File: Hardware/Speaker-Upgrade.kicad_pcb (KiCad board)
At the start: 2 copper layers, 130.2 x 56.5 mm, 33 parts, among them J1 POWER, J2 CONN_PCB1, J3 CONN_PCB2, J4 AUDIO_JACK, U1 LM7805, U2 WIN-668, U3 AN7522N

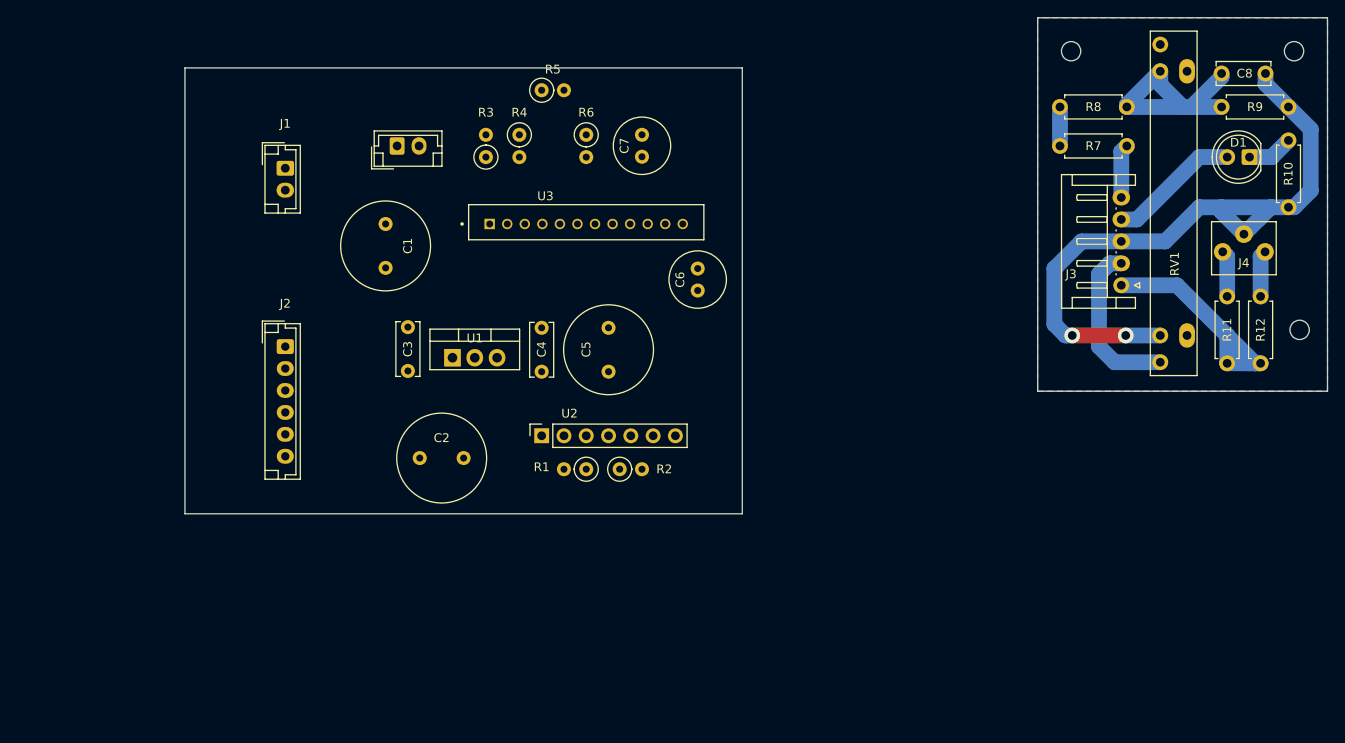
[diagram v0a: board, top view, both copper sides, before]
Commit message: Improvements on schematics and PCB
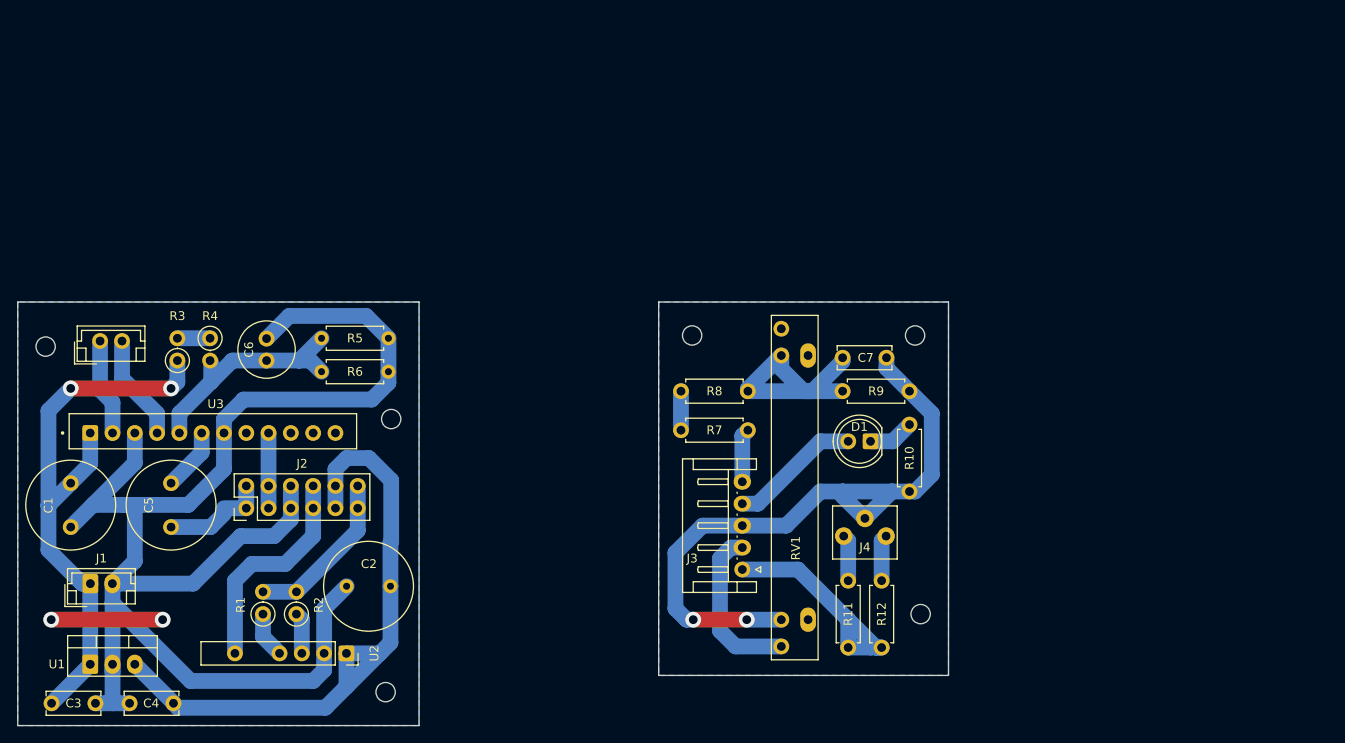
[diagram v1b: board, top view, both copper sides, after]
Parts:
- removed the C5 at (162.6, 72.7)
- added H1: MountingHole, MountingHole:MountingHole_2.2mm_M2, F.Cu at (98.4, 69.8)
- added H2: MountingHole, MountingHole:MountingHole_2.2mm_M2, F.Cu at (137.8, 78.1)
- added H3: MountingHole, MountingHole:MountingHole_2.2mm_M2, F.Cu at (137.2, 109.2)
- C2: value 1000uF -> 2200uF; footprint Capacitor_THT:C_Radial_D10.0mm_H12.5mm_P5.00mm -> Capacitor_THT:C_Radial_D10.0mm_H16.0mm_P5.00mm
- C5: renamed from C6; footprint Capacitor_THT:C_Radial_D6.3mm_H11.0mm_P2.50mm -> Capacitor_THT:C_Radial_D10.0mm_H16.0mm_P5.00mm
- J2: footprint Connector_JST:JST_EH_B6B-EH-A_1x06_P2.50mm_Vertical -> Connector_PinHeader_2.54mm:PinHeader_2x06_P2.54mm_Vertical
- R5, R6: footprint Resistor_THT:R_Axial_DIN0207_L6.3mm_D2.5mm_P2.54mm_Vertical -> Resistor_THT:R_Axial_DIN0207_L6.3mm_D2.5mm_P7.62mm_Horizontal
- moved C5 64.8 mm to (112.7, 85.4)
- moved C4 56.5 mm to (113.0, 110.5), turned to 180 degrees
- moved C3 55.5 mm to (99.1, 110.5), turned to 0 degrees
- moved U1 54.1 mm to (103.5, 106.0)
- moved C7 54.0 mm to (189.2, 71.1)
- moved D1 54.0 mm to (192.4, 80.6)
- moved H6 54.0 mm to (198.1, 100.3)
- moved R10 54.0 mm to (196.8, 86.4)
- moved R7 54.0 mm to (178.4, 79.4)
- moved R8 54.0 mm to (170.8, 74.9)
- moved R9 54.0 mm to (189.2, 74.9)
- moved RV1 54.0 mm to (183.9, 86.0)
- moved H4 54.0 mm to (172.1, 68.6)
- moved H5 54.0 mm to (197.5, 68.6)
- moved J3 54.0 mm to (177.8, 95.2)
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- renumbered C7 to C6, C8 to C7, H1 to H4, H2 to H5, H3 to H6
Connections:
- net PCB2_5V renamed UI_5V
- net PCB2_AUDIO renamed UI_AUDIO
- net PCB2_GND renamed UI_GND
- net PCB2_LED renamed UI_LED
- net PCB2_VOL renamed UI_VOLUME
- J2 pad 1: +5V -> MAIN_AUDIO
- J2 pad 2: GND -> VOLUME
- J2 pad 3: VOLUME -> GND
- J2 pad 5: BT_AUDIO -> +5V
- J2 pad 6: MAIN_AUDIO -> BT_AUDIO
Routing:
- net GND: track 0.00 -> 184.9 mm, vias 0 -> 2
- net +5V: track 0.00 -> 72.8 mm
- net +12V: track 0.00 -> 66.4 mm, vias 0 -> 2
- net STAND_BY: track 0.00 -> 27.2 mm
- net LED: track 0.00 -> 25.0 mm
- net BT_AUDIO: track 0.00 -> 18.8 mm
- net CH1_OUT(-): track 0.00 -> 12.1 mm
- net MAIN_AUDIO: track 0.00 -> 11.7 mm
- net CH1_OUT(+): track 0.00 -> 11.1 mm
- net VOLUME: track 0.00 -> 8.57 mm
- net CH1_IN: track 0.00 -> 7.16 mm
- net BT_LEFT: track 0.00 -> 5.25 mm
- net BT_RIGHT: track 0.00 -> 4.74 mm
- net Net-(R3-Pad2): track 0.00 -> 3.72 mm
- added copper zone on B.Cu, net GND
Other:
- board size 130.2 x 56.5 mm -> 106 x 48.3 mm

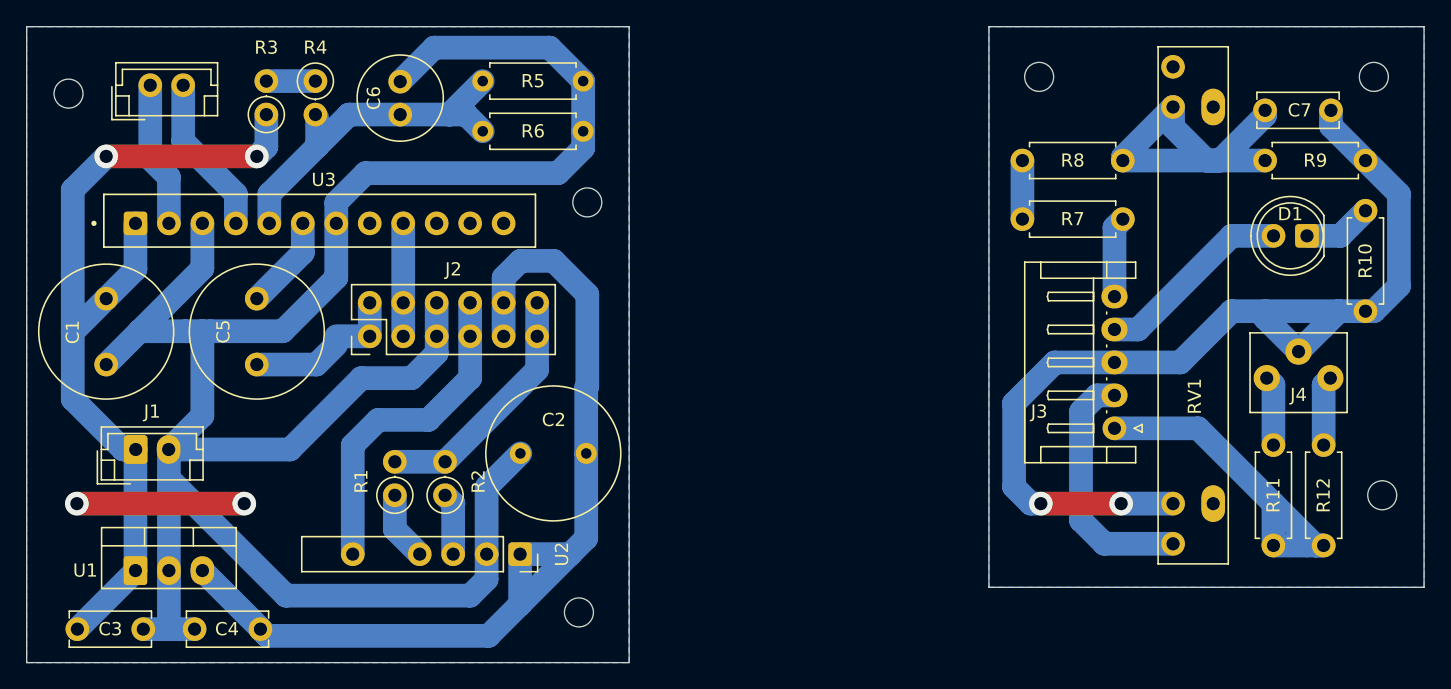
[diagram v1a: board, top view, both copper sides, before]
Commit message: Improvements on schematics and PCB
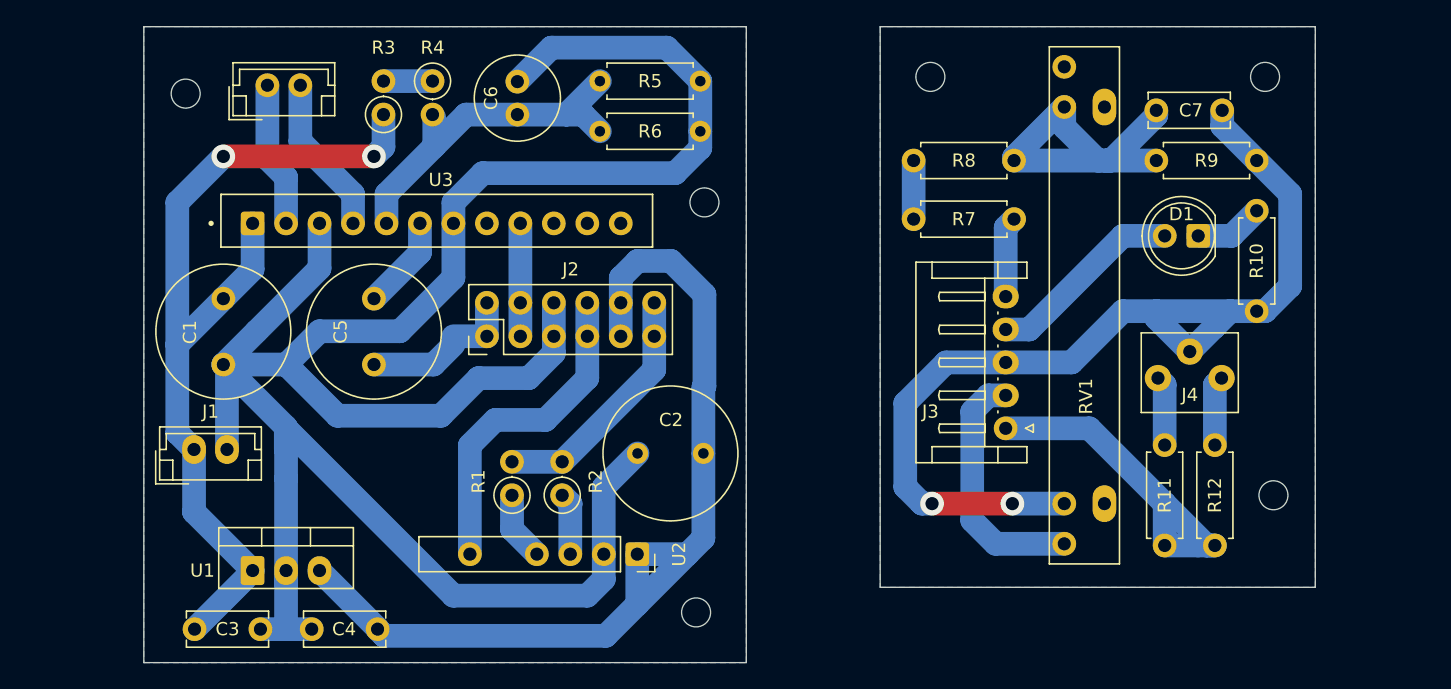
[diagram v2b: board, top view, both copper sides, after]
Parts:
- moved H2 8.89 mm to (146.7, 78.1)
- moved H3 8.89 mm to (146.1, 109.2)
- moved J2 8.89 mm to (130.2, 88.3)
- moved R2 8.89 mm to (132.1, 100.3)
- moved R5 8.89 mm to (146.4, 68.9)
- moved R6 8.89 mm to (146.4, 72.7)
- moved U2 8.89 mm to (141.6, 104.8)
- moved C1 8.89 mm to (110.2, 85.4)
- moved C3 8.89 mm to (108.0, 110.5)
- moved C4 8.89 mm to (121.9, 110.5)
- moved C5 8.89 mm to (121.6, 85.4)
- moved C6 8.89 mm to (132.5, 71.4)
- moved H1 8.89 mm to (107.3, 69.8)
- moved LS1 8.89 mm to (113.5, 69.2)
- moved R3 8.89 mm to (122.3, 71.4)
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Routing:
- net GND: track 184.9 -> 182.9 mm, vias 2 -> 0
- net +12V: track 66.4 -> 68.0 mm
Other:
- board size 106 x 48.3 mm -> 88.9 x 48.3 mm
